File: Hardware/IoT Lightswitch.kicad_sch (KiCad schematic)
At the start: 23 parts, among them J1 Screw_Terminal_01x04, J2 Conn_01x04, K1 SANYOU_SRD_Form_C, Q1 NMOS, SW1 SW_SPDT, SW2 SW_SPDT, SW3 SW_Push, SW4 SW_Push, SW5 SW_SPST, U1 ESP32-S2-SOLO-2

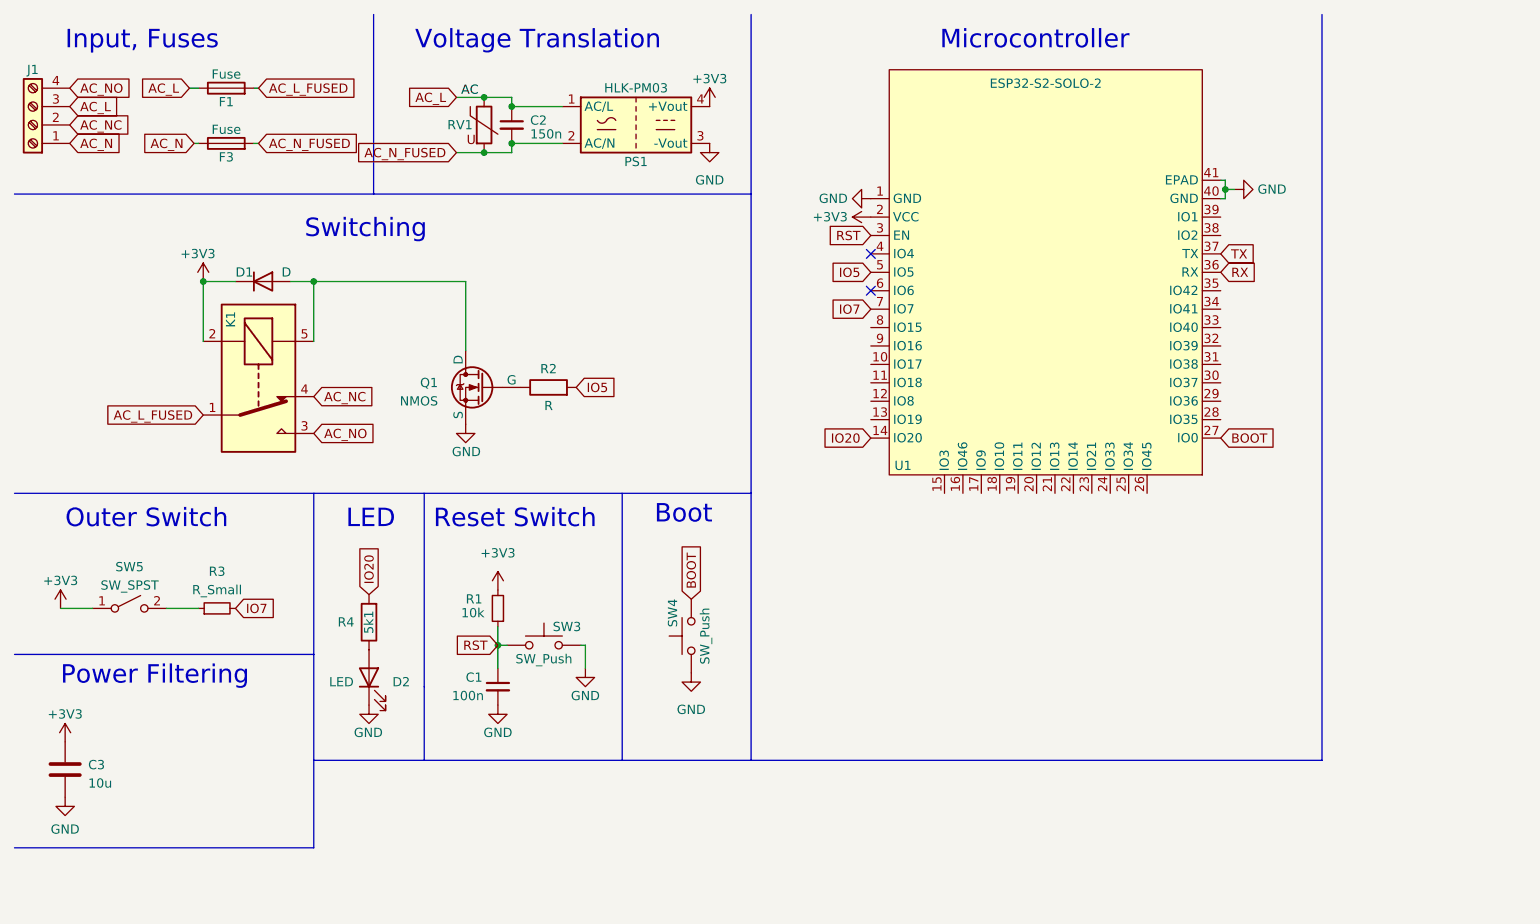
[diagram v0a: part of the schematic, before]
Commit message: Updated Schema
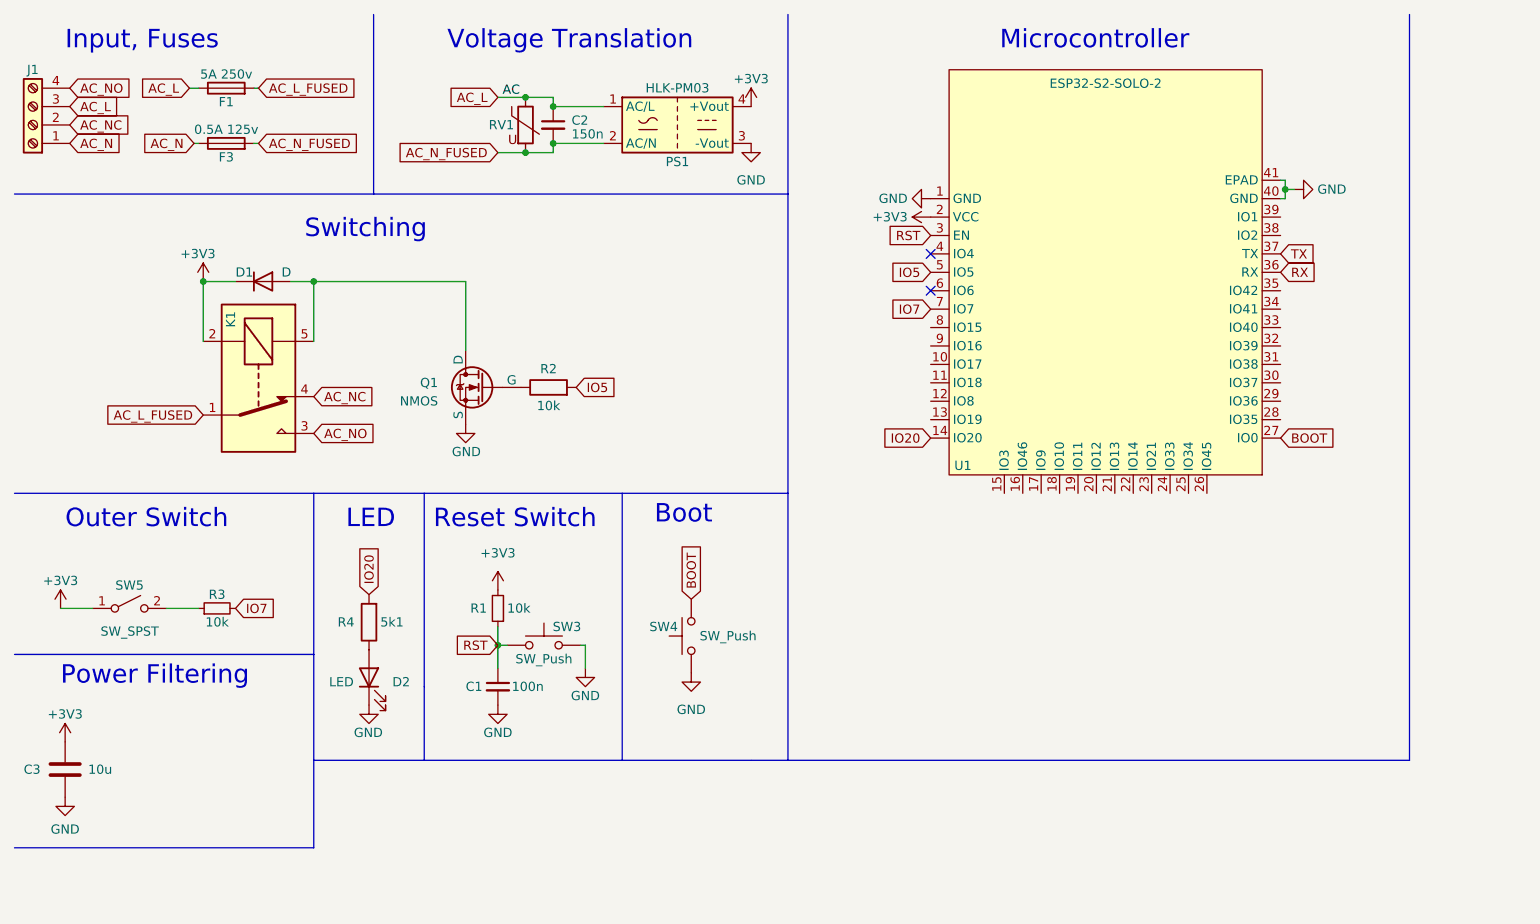
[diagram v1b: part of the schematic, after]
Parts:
- C2: Rating (none) -> 250v
- F1: value Fuse -> 5A 250v
- F3: value Fuse -> 0.5A 125v
- R2: value R -> 10k
- R3: value R_Small -> 10k
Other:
- moved on the sheet: C2, PS1, RV1, U1
